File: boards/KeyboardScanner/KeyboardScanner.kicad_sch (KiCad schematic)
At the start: 20 parts, among them J1 Keyboard1, J2 Keyboard1, J3 Encoder, J4 Select, U5 ULN2803A, U8 4069

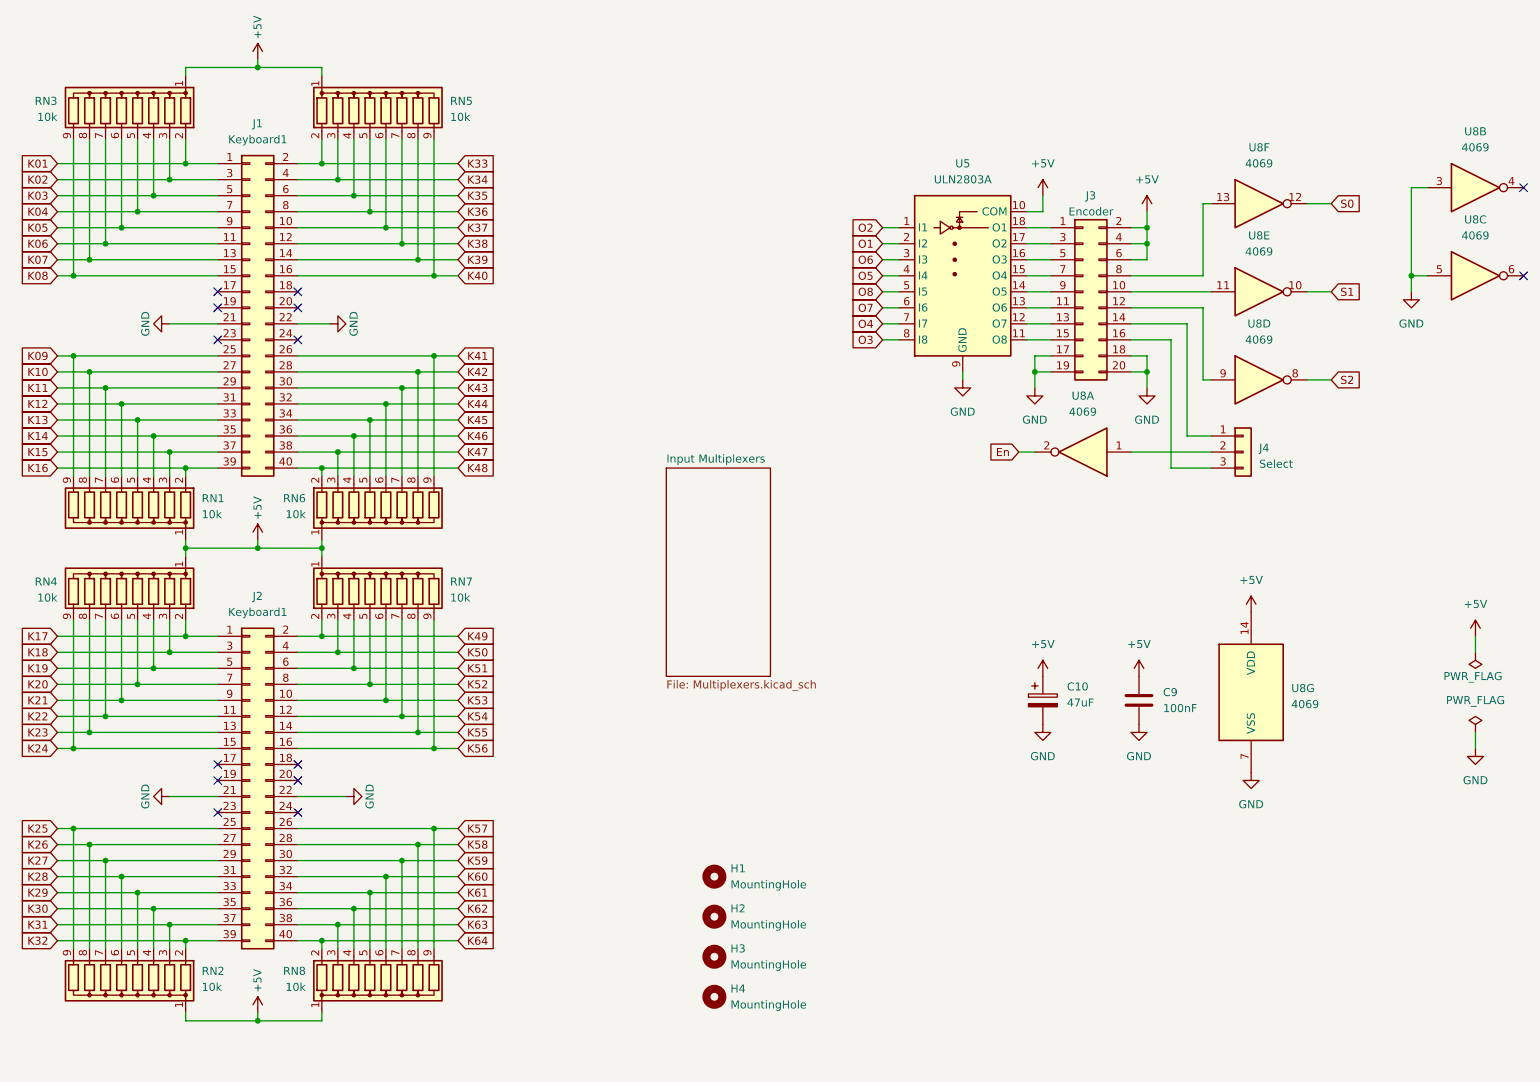
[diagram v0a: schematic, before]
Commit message: Revert "Reverting to using 2803A inverted open collector for Keyboard Scanner, fixed layout"
This reverts commit 7b46a6886eac97662925cbadd02de0ff96663bd2.
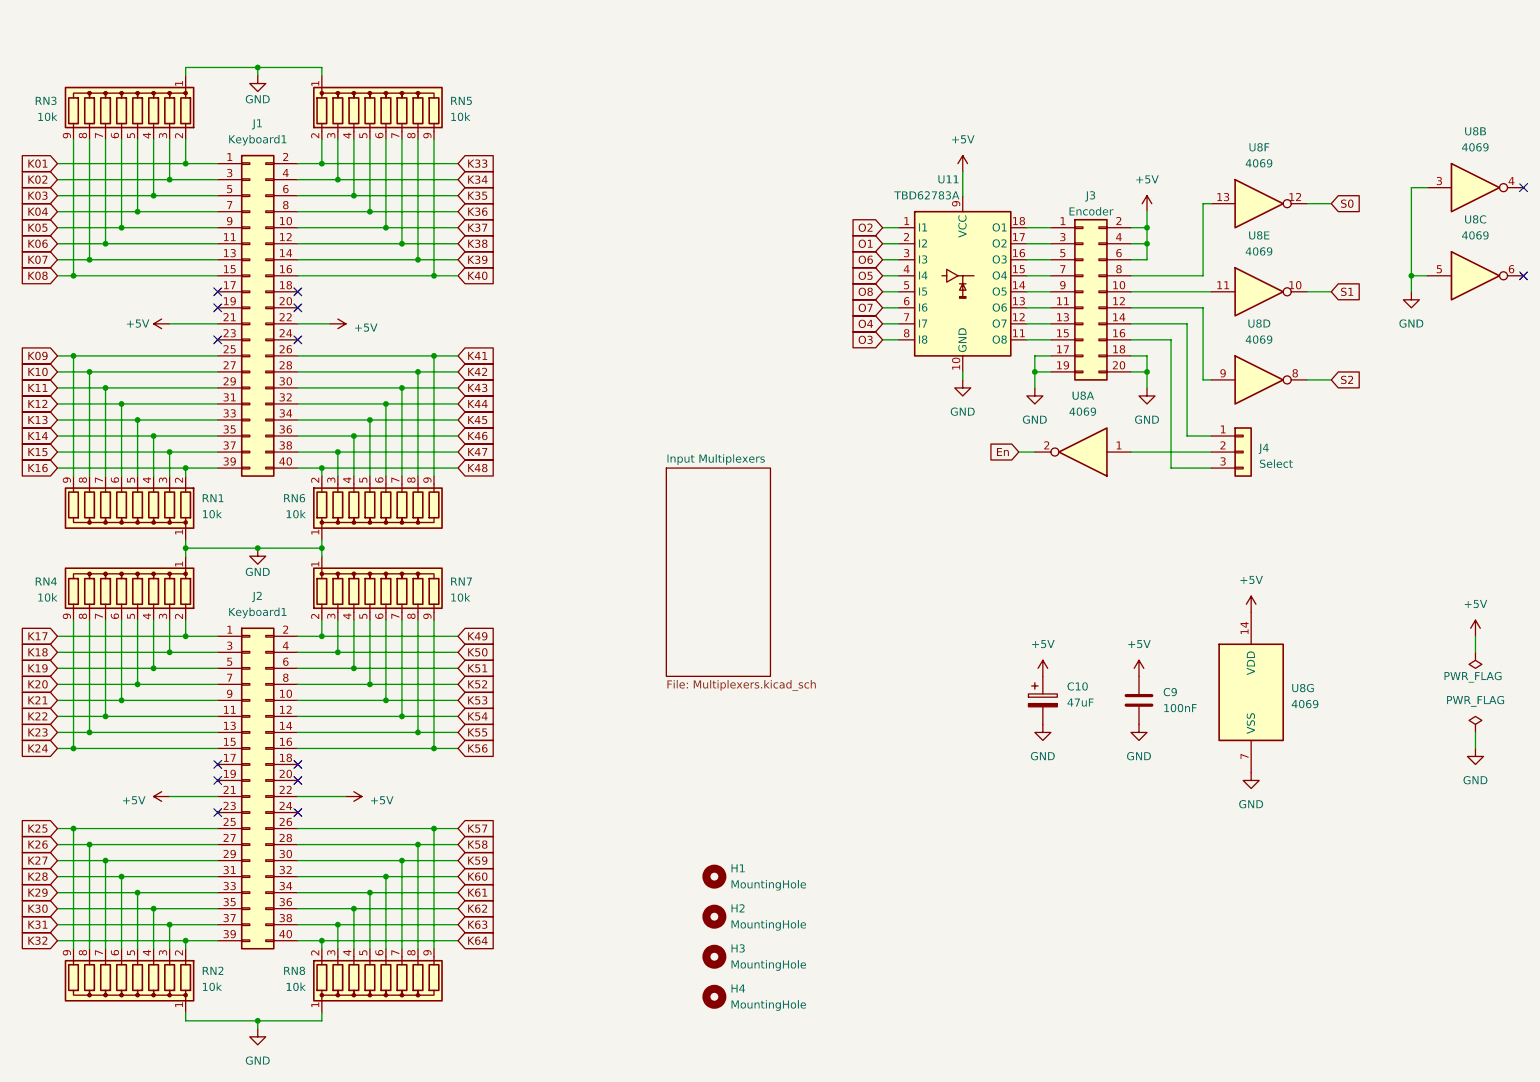
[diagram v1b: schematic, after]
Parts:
- removed U5: ULN2803A, Package_DIP:DIP-18_W7.62mm, symbol Transistor_Array:ULN2803A
- added U11: TBD62783A, Package_DIP:DIP-18_W7.62mm, symbol Transistor_Array:TBD62783A
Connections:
- net +5V: now also J1.21 (Pin_21), J1.22 (Pin_22), J2.21 (Pin_21), J2.22 (Pin_22), U11.9 (VCC); no longer RN1.1 (common), RN2.1 (common), RN3.1 (common), RN4.1 (common), RN5.1 (common), RN6.1 (common), RN7.1 (common), RN8.1 (common)
- net GND: now also RN1.1 (common), RN2.1 (common), RN3.1 (common), RN4.1 (common), RN5.1 (common), RN6.1 (common), RN7.1 (common), RN8.1 (common), U11.10 (GND); no longer J1.21 (Pin_21), J1.22 (Pin_22), J2.21 (Pin_21), J2.22 (Pin_22)
- net O1: now also U11.2 (I2)
- net O2: now also U11.1 (I1)
- net O3: now also U11.8 (I8)
- net O4: now also U11.7 (I7)
- net O5: now also U11.4 (I4)
- net O6: now also U11.3 (I3)
- net O7: now also U11.6 (I6)
- net O8: now also U11.5 (I5)
- net at J3.1 (Pin_1): now also U11.18 (O1)
- net at J3.11 (Pin_11): now also U11.13 (O6)
- net at J3.13 (Pin_13): now also U11.12 (O7)
- net at J3.15 (Pin_15): now also U11.11 (O8)
- net at J3.3 (Pin_3): now also U11.17 (O2)
- net at J3.5 (Pin_5): now also U11.16 (O3)
- net at J3.7 (Pin_7): now also U11.15 (O4)
- net at J3.9 (Pin_9): now also U11.14 (O5)

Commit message: Reverting to using 2803A inverted open collector for Keyboard Scanner, fixed layout
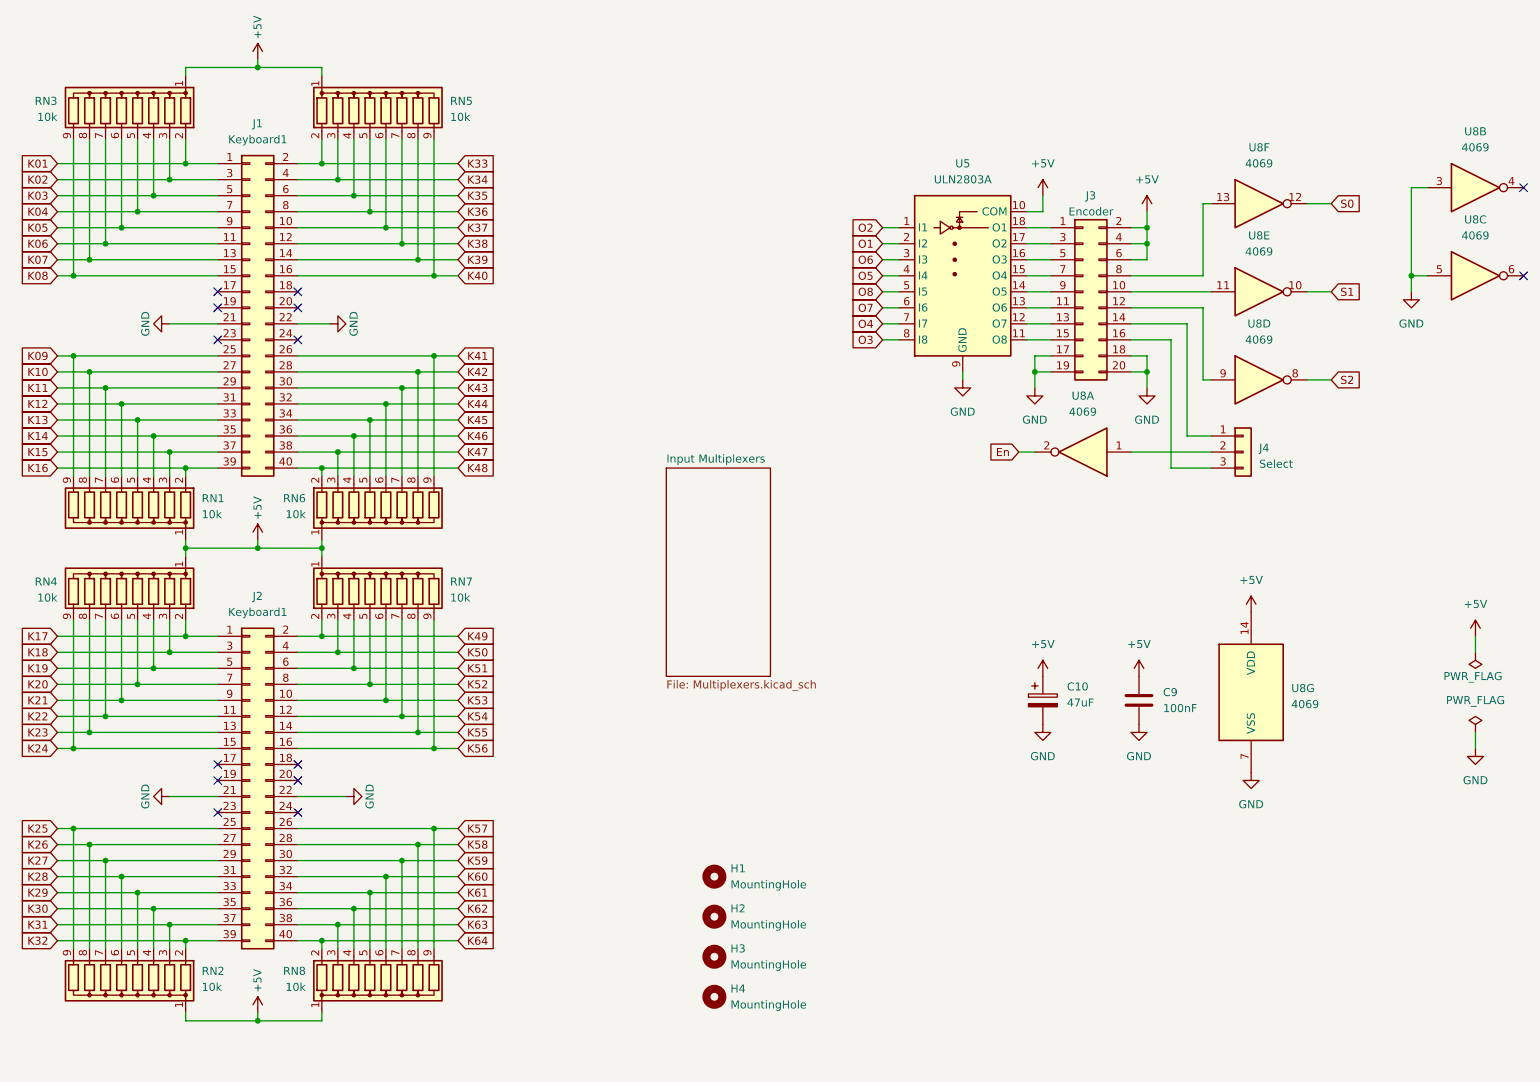
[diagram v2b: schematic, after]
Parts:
- removed U11: TBD62783A, Package_DIP:DIP-18_W7.62mm, symbol Transistor_Array:TBD62783A
- added U5: ULN2803A, Package_DIP:DIP-18_W7.62mm, symbol Transistor_Array:ULN2803A
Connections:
- net +5V: now also RN1.1 (common), RN2.1 (common), RN3.1 (common), RN4.1 (common), RN5.1 (common), RN6.1 (common), RN7.1 (common), RN8.1 (common), U5.10 (COM); no longer J1.21 (Pin_21), J1.22 (Pin_22), J2.21 (Pin_21), J2.22 (Pin_22)
- net GND: now also J1.21 (Pin_21), J1.22 (Pin_22), J2.21 (Pin_21), J2.22 (Pin_22), U5.9 (GND); no longer RN1.1 (common), RN2.1 (common), RN3.1 (common), RN4.1 (common), RN5.1 (common), RN6.1 (common), RN7.1 (common), RN8.1 (common)
- net O1: now also U5.2 (I2)
- net O2: now also U5.1 (I1)
- net O3: now also U5.8 (I8)
- net O4: now also U5.7 (I7)
- net O5: now also U5.4 (I4)
- net O6: now also U5.3 (I3)
- net O7: now also U5.6 (I6)
- net O8: now also U5.5 (I5)
- net at J3.1 (Pin_1): now also U5.18 (O1)
- net at J3.11 (Pin_11): now also U5.13 (O6)
- net at J3.13 (Pin_13): now also U5.12 (O7)
- net at J3.15 (Pin_15): now also U5.11 (O8)
- net at J3.3 (Pin_3): now also U5.17 (O2)
- net at J3.5 (Pin_5): now also U5.16 (O3)
- net at J3.7 (Pin_7): now also U5.15 (O4)
- net at J3.9 (Pin_9): now also U5.14 (O5)
